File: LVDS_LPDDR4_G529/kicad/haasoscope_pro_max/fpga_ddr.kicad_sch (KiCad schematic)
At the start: 2 parts, among them U1 MT53D512M16D1DS_Aligned, U3 Ti90G529_Functions

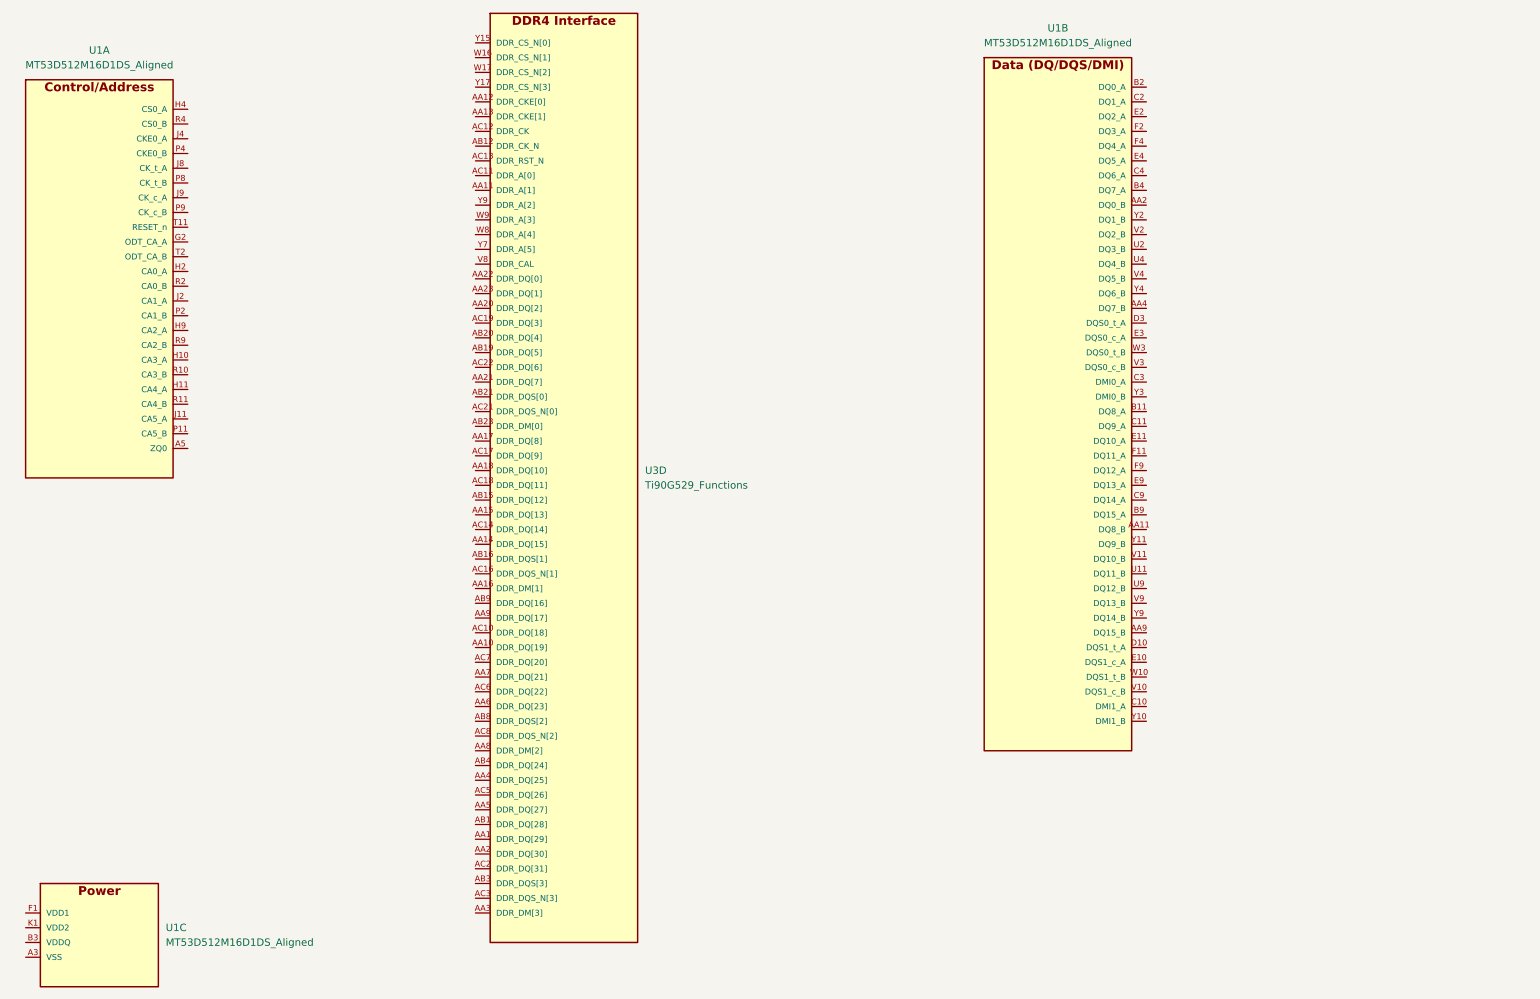
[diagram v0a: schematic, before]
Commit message: Aligned schematics, sort of
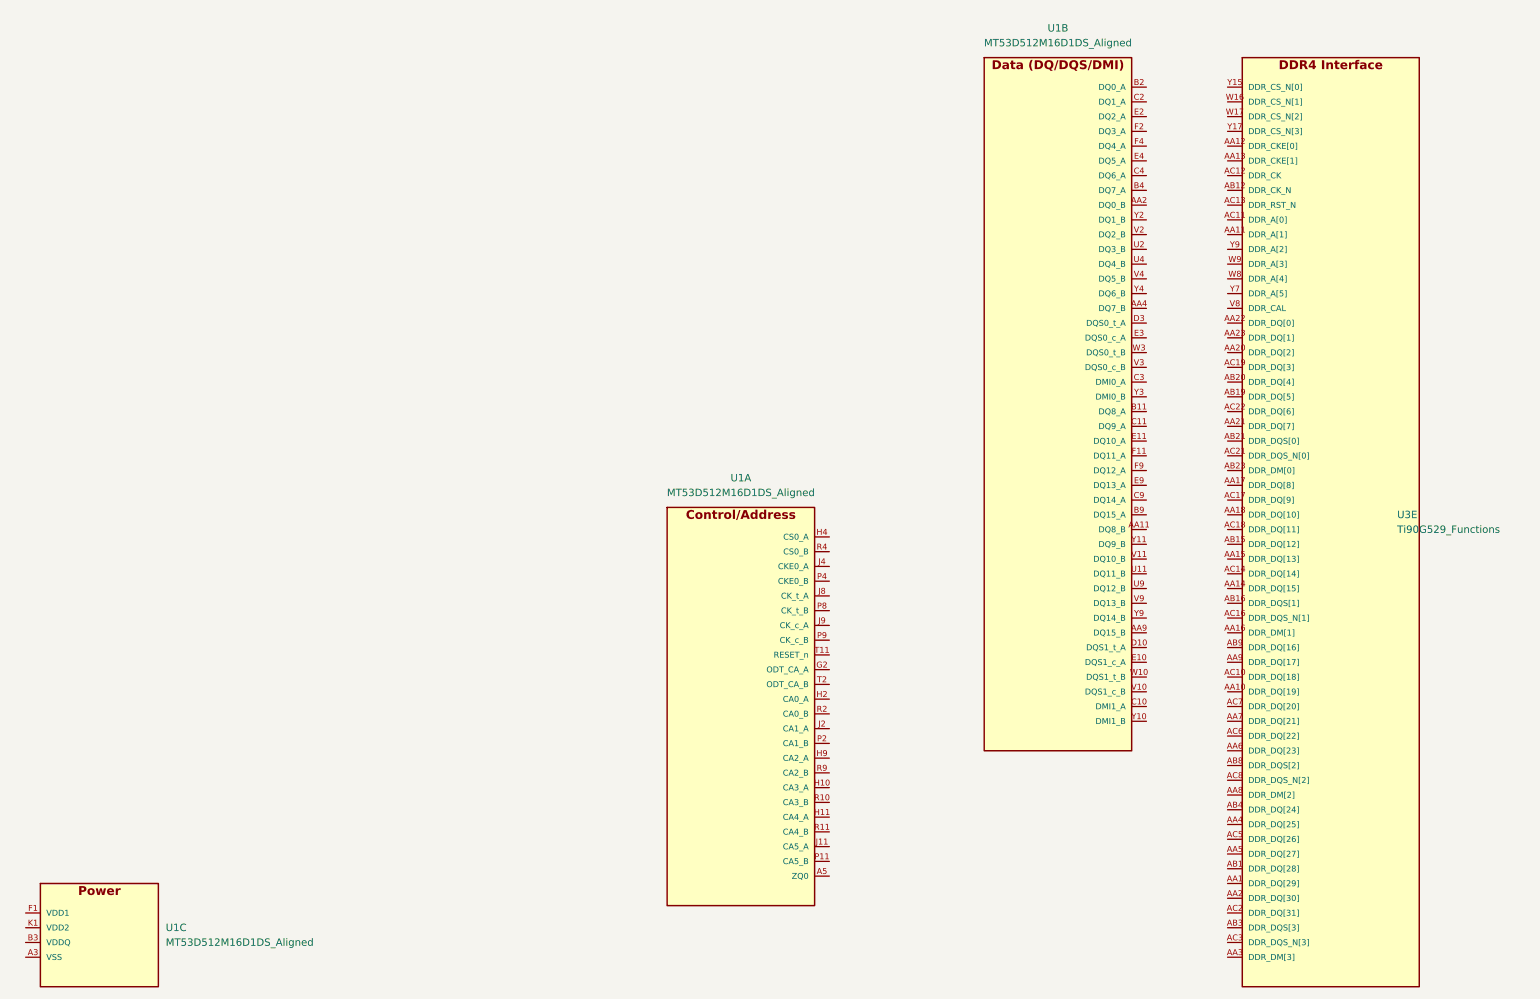
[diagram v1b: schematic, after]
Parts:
- removed U3: Ti90G529_Functions, G529:BGA-529_23x23_19.0x19.0mm, symbol Ti90G529_Functions:Ti90G529_Functions
- added U3: Ti90G529_Functions, haasoscope_pro_adc_fpga_board:BGA-529_23x23_19.0x19.0mm, symbol Ti90G529_Functions:Ti90G529_Functions
- U1: footprint MT53D512M32D2DS-053 WT_D:IC_MT53D512M16D1DS-046_WT_D -> easyeda2kicad:WFBGA-200_L14.5-W10.0-BL_MT53D512M32D2DS
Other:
- moved on the sheet: U1A
